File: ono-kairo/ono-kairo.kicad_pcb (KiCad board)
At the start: 2 copper layers, 20 parts, among them J1 Conn_02x01, J2 Conn_02x02_Top_Bottom, U1 MCP3208, U2 DS18B20, U3 MCP6002-xMC

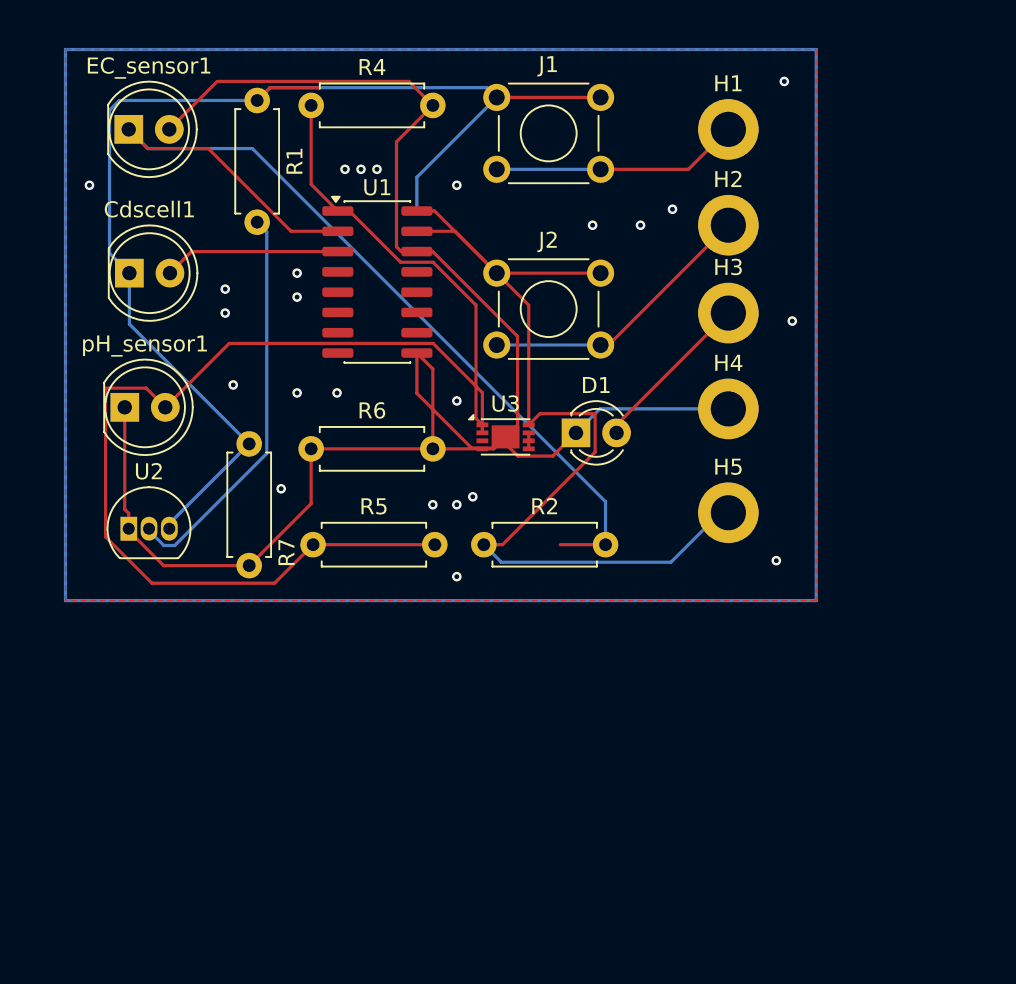
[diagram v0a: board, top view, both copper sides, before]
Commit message: Add files via upload
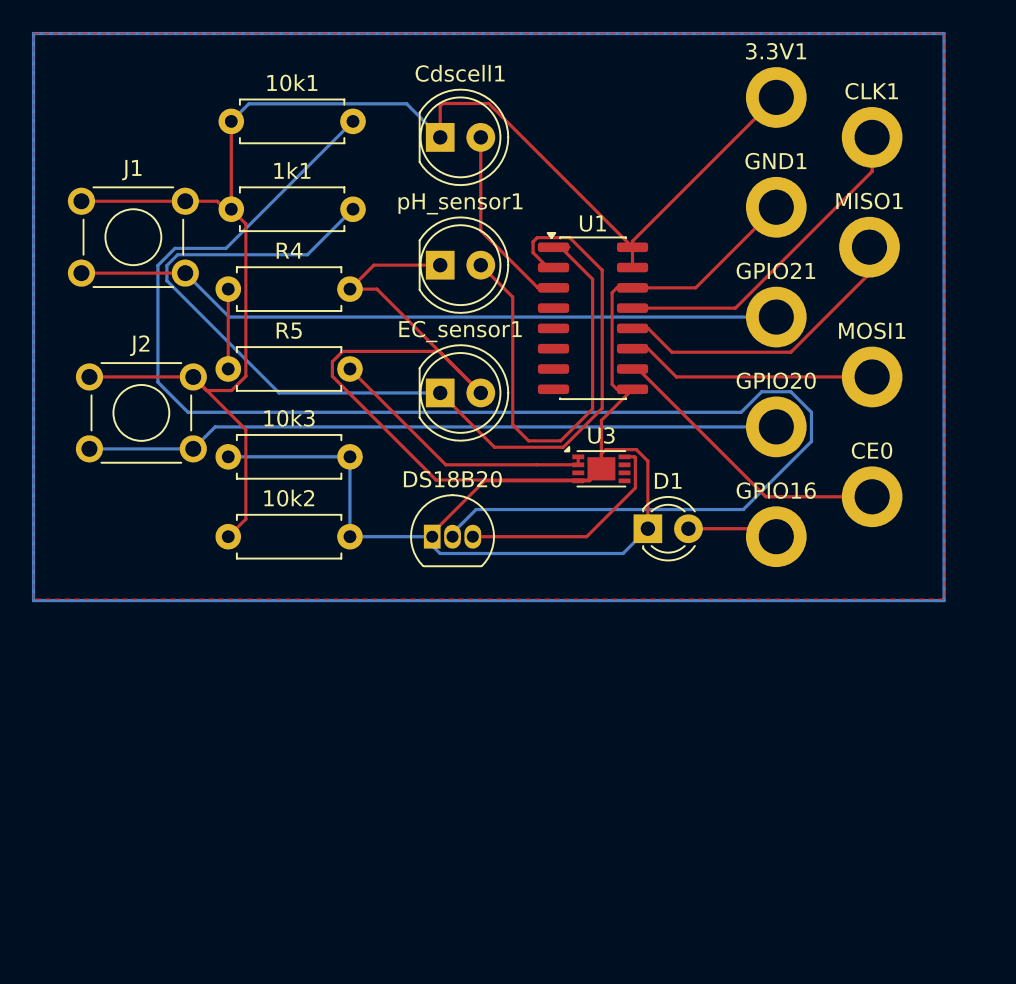
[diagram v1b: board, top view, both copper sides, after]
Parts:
- removed H1: gpio21, MountingHole:MountingHole_2.2mm_M2_DIN965_Pad
- removed H2: gpio20, MountingHole:MountingHole_2.2mm_M2_DIN965_Pad
- removed H3: gpio16, MountingHole:MountingHole_2.2mm_M2_DIN965_Pad
- removed H4: GND, MountingHole:MountingHole_2.2mm_M2_DIN965_Pad
- removed H5: 3.3V, MountingHole:MountingHole_2.2mm_M2_DIN965_Pad
- removed R1, R6, R7: 10k, Resistor_THT:R_Axial_DIN0207_L6.3mm_D2.5mm_P7.62mm_Horizontal
- removed R2: 1k, Resistor_THT:R_Axial_DIN0207_L6.3mm_D2.5mm_P7.62mm_Horizontal
- removed U2: DS18B20, Package_TO_SOT_THT:TO-92_Inline
- added 10k1: 10k, Resistor_THT:R_Axial_DIN0207_L6.3mm_D2.5mm_P7.62mm_Horizontal, F.Cu at (153.4, 35.0)
- added 10k2: 10k, Resistor_THT:R_Axial_DIN0207_L6.3mm_D2.5mm_P7.62mm_Horizontal, F.Cu at (153.2, 61.0)
- added 10k3: 10k, Resistor_THT:R_Axial_DIN0207_L6.3mm_D2.5mm_P7.62mm_Horizontal, F.Cu at (153.2, 56.0)
- added 1k1: 1k, Resistor_THT:R_Axial_DIN0207_L6.3mm_D2.5mm_P7.62mm_Horizontal, F.Cu at (153.4, 40.5)
- added 3.3V1: 3.3V, MountingHole:MountingHole_2.2mm_M2_DIN965_Pad, F.Cu at (187.5, 33.5)
- added CE0: CE0, MountingHole:MountingHole_2.2mm_M2_DIN965_Pad, F.Cu at (193.5, 58.5)
- added CLK1: CLK, MountingHole:MountingHole_2.2mm_M2_DIN965_Pad, F.Cu at (193.5, 36.0)
- added DS18B20: DS18B20, Package_TO_SOT_THT:TO-92_Inline, F.Cu at (166.0, 61.0)
- added GND1: GND, MountingHole:MountingHole_2.2mm_M2_DIN965_Pad, F.Cu at (187.5, 40.4)
- added GPIO16: gpio16, MountingHole:MountingHole_2.2mm_M2_DIN965_Pad, F.Cu at (187.5, 61.0)
- added GPIO20: gpio20, MountingHole:MountingHole_2.2mm_M2_DIN965_Pad, F.Cu at (187.5, 54.1)
- added GPIO21: gpio21, MountingHole:MountingHole_2.2mm_M2_DIN965_Pad, F.Cu at (187.5, 47.2)
- added MISO1: MISO, MountingHole:MountingHole_2.2mm_M2_DIN965_Pad, F.Cu at (193.3, 42.9)
- added MOSI1: MOSI, MountingHole:MountingHole_2.2mm_M2_DIN965_Pad, F.Cu at (193.5, 51.0)
- J2: value Conn_02x02_Top_Bottom -> 02x02_Bottom
- moved J1 26.8 mm to (144.0, 40.0)
- moved J2 26.3 mm to (144.5, 51.0)
- moved EC_sensor1 25.5 mm to (166.5, 52.0)
- moved pH_sensor1 21.7 mm to (166.5, 44.0)
- moved Cdscell1 21.2 mm to (166.5, 36.0)
- moved U1 13.7 mm to (176.0, 47.3)
- moved R4 12.6 mm to (153.2, 45.5)
- moved R5 12.2 mm to (153.2, 50.5)
- moved D1 7.50 mm to (179.5, 60.5)
- moved U3 6.32 mm to (176.6, 56.8)
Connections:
- U1 pad 10: CE0 -> Net-(U1-~{CS}/SHDN)
- U1 pad 11: MOSI -> Net-(U1-Din)
- U1 pad 12: MISO -> Net-(U1-Dout)
- U1 pad 13: CLK -> Net-(U1-CLK)
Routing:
- net Net-(DS18B20-DQ): track 0.00 -> 92.9 mm
- net Net-(U1-CH0): track 88.2 -> 51.7 mm
- net Net-(DS18B20-V_{DD}): track 139.5 -> 108.9 mm
- net Net-(J1-Pin_2): track 15.5 -> 44.6 mm
- net Net-(J2-Pin_2): track 17.6 -> 43.6 mm
- net Net-(U2-DQ): track 25.0 -> 0.00 mm
- net Net-(U1-CLK): track 0.00 -> 20.7 mm
- net Net-(U1-Dout): track 0.00 -> 19.1 mm
- net Net-(U1-~{CS}/SHDN): track 0.00 -> 18.3 mm
- net Net-(U1-Din): track 0.00 -> 15.7 mm
- net Net-(D1-K): track 114.4 -> 127.6 mm
- net Net-(D1-A): track 10.4 -> 5.71 mm
- net Net-(U1-CH1): track 61.1 -> 62.9 mm
- net (no net): track 1.00 -> 0.00 mm, vias 24 -> 0
- net Net-(U1-CH2): track 11.1 -> 11.9 mm

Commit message: Add files via upload
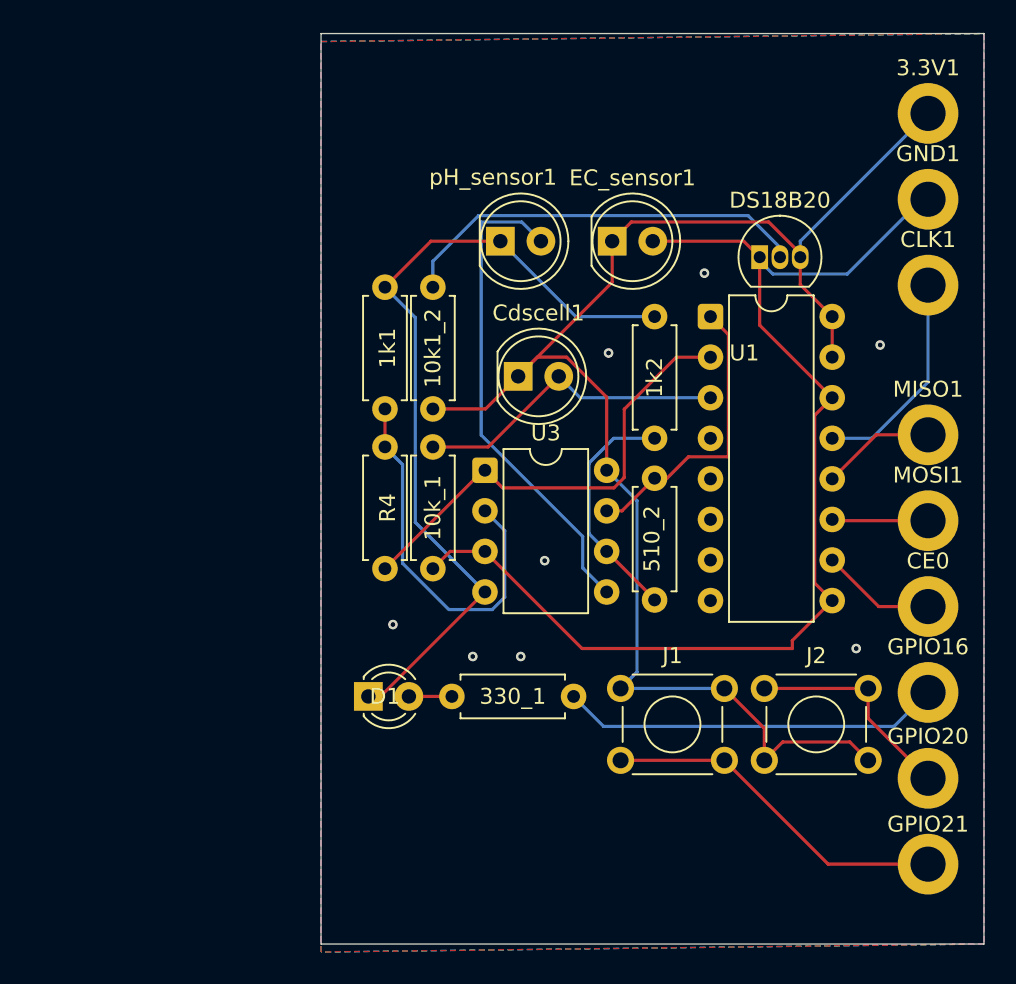
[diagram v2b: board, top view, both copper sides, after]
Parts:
- removed 10k1, 10k2, 10k3: 10k, Resistor_THT:R_Axial_DIN0207_L6.3mm_D2.5mm_P7.62mm_Horizontal
- removed R5: 1M, Resistor_THT:R_Axial_DIN0207_L6.3mm_D2.5mm_P7.62mm_Horizontal
- added 10k1_2: 10k, Resistor_THT:R_Axial_DIN0207_L6.3mm_D2.5mm_P7.62mm_Horizontal, F.Cu at (166.0, 53.0)
- added 10k_1: 10k, Resistor_THT:R_Axial_DIN0207_L6.3mm_D2.5mm_P7.62mm_Horizontal, F.Cu at (166.0, 55.4)
- added 1k2: 1k, Resistor_THT:R_Axial_DIN0207_L6.3mm_D2.5mm_P7.62mm_Horizontal, F.Cu at (179.9, 54.8)
- added 330_1: 330, Resistor_THT:R_Axial_DIN0207_L6.3mm_D2.5mm_P7.62mm_Horizontal, F.Cu at (167.2, 71.0)
- added 510_2: 510, Resistor_THT:R_Axial_DIN0207_L6.3mm_D2.5mm_P7.62mm_Horizontal, F.Cu at (179.9, 57.3)
- J1: value Conn_02x01 -> Conn
- J2: value 02x02_Bottom -> Bottom
- U1: footprint Package_SO:SOIC-16_3.9x9.9mm_P1.27mm -> Package_DIP:DIP-16_W7.62mm
- U3: footprint Package_DFN_QFN:DFN-8-1EP_3x2mm_P0.5mm_EP1.75x1.45mm -> Package_DIP:DIP-8_W7.62mm
- moved J2 46.5 mm to (186.8, 70.5)
- moved J1 45.5 mm to (177.8, 70.5)
- moved GPIO21 35.5 mm to (197.0, 81.5)
- moved DS18B20 27.0 mm to (186.5, 43.5)
- moved GPIO20 24.0 mm to (197.0, 76.1)
- moved D1 20.4 mm to (162.0, 71.0)
- moved R4 20.1 mm to (163.0, 63.0), turned to 90 degrees
- moved 1k1 15.8 mm to (163.0, 53.0), turned to 90 degrees
- moved Cdscell1 15.7 mm to (171.3, 51.0)
- moved EC_sensor1 14.4 mm to (177.2, 42.5)
- moved GPIO16 13.6 mm to (197.0, 70.7)
- moved MISO1 12.3 mm to (197.0, 54.6)
- moved CLK1 9.89 mm to (197.0, 45.3)
- moved MOSI1 9.65 mm to (197.0, 60.0)
- moved 3.3V1 9.55 mm to (197.0, 34.5)
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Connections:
- 1k1 pad 1: Net-(DS18B20-V_{DD}) -> Net-(U3A--)
- 1k1 pad 2: Net-(U1-CH1) -> Net-(D1-K)
- EC_sensor1 pad 1: Net-(U1-CH1) -> Net-(DS18B20-V_{DD})
- GPIO16 pad 1: Net-(D1-A) -> Net-(330_1-Pad2)
- GPIO20 pad 1: Net-(J2-Pin_2) -> Net-(J2-Pin_1)
- J2 pad 1: Net-(DS18B20-V_{DD}) -> Net-(J2-Pin_1)
- J2 pad 2: Net-(J2-Pin_2) -> Net-(DS18B20-V_{DD})
- R4 pad 1: Net-(U1-CH0) -> Net-(U1-CH1)
- R4 pad 2: Net-(D1-K) -> Net-(U3A--)
- U3 pad 1: Net-(U1-CH0) -> Net-(U1-CH1)
- U3 pad 2: Net-(U1-CH0) -> Net-(U3A--)
- U3 pad 3: unconnected-(U3A-+-Pad3) -> Net-(D1-K)
- U3 pad 5: (no net) -> Net-(U3B-+)
- U3 pad 6: (no net) -> Net-(U3B--)
- U3 pad 7: (no net) -> Net-(U1-CH0)
- pH_sensor1 pad 2: Net-(U1-CH0) -> Net-(U3B-+)
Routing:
- net Net-(DS18B20-DQ): track 92.9 -> 26.0 mm
- net Net-(J2-Pin_2): track 43.6 -> 0.00 mm
- net Net-(U1-CH1): track 62.9 -> 29.3 mm
- net Net-(U1-CH0): track 51.7 -> 18.3 mm
- net Net-(U3B-+): track 0.00 -> 30.7 mm
- net Net-(U3A--): track 0.00 -> 24.0 mm
- net Net-(330_1-Pad2): track 0.00 -> 23.8 mm
- net Net-(J1-Pin_2): track 44.6 -> 21.9 mm
- net Net-(U3B--): track 0.00 -> 15.0 mm
- net Net-(J2-Pin_1): track 0.00 -> 13.7 mm
- net Net-(DS18B20-V_{DD}): track 108.9 -> 96.5 mm
- net Net-(U1-Dout): track 19.1 -> 7.14 mm
- net Net-(U1-~{CS}/SHDN): track 18.3 -> 7.21 mm
- net Net-(U1-Din): track 15.7 -> 6.03 mm
- net Net-(U1-CH2): track 11.9 -> 19.8 mm
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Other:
- board outline added: 41.5 x 57 mm
